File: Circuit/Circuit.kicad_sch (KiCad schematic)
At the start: 21 parts, among them SW1 SW_DPDT_x2, SW2 SW_DPDT_x2, SW3 SW_DPDT_x2, U1 L7805

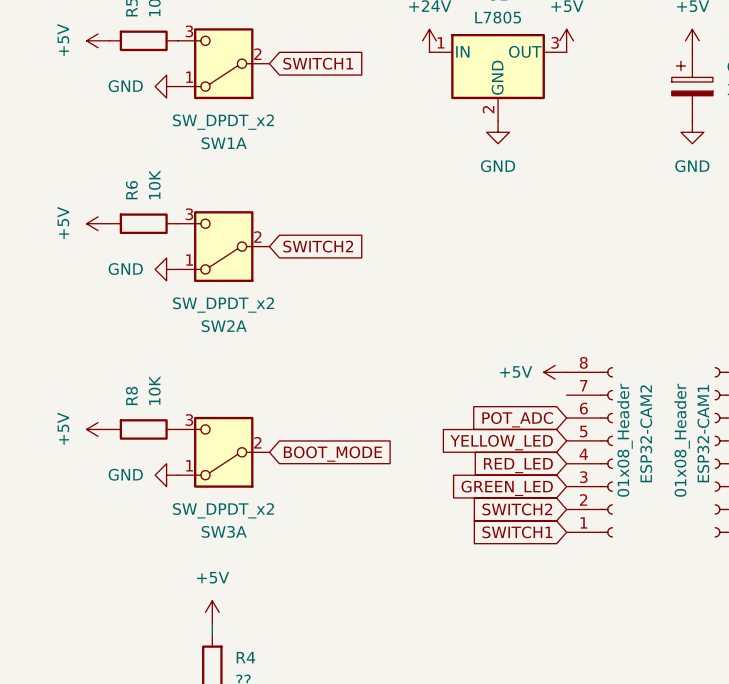
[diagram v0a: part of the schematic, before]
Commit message: fixed PCB, started programming
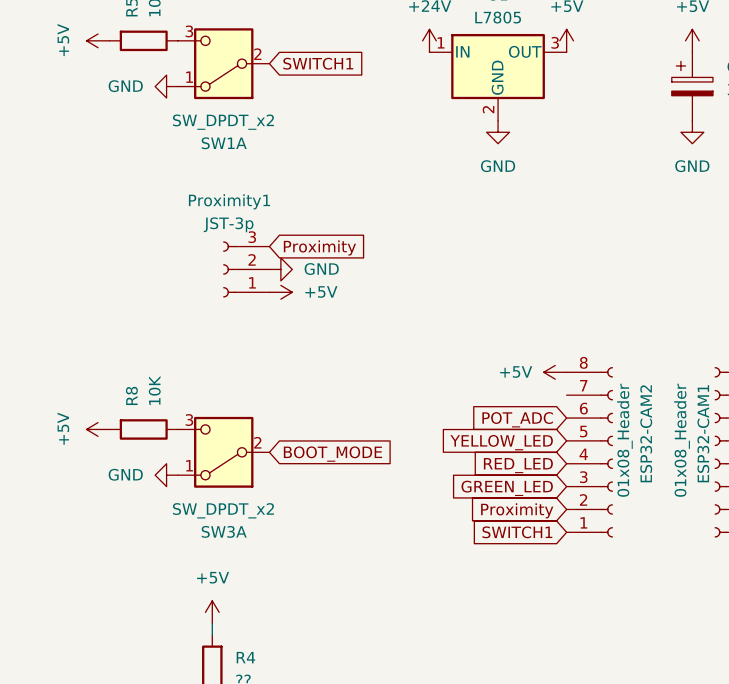
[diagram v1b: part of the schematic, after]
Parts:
- removed R6: 10K, Resistor_THT:R_Axial_DIN0207_L6.3mm_D2.5mm_P7.62mm_Horizontal, symbol Device:R
- removed SW2: SW_DPDT_x2, Connector_PinSocket_2.54mm:PinSocket_1x03_P2.54mm_Vertical, symbol Switch:SW_DPDT_x2
- added Proximity1: JST-3p, Connector_JST:JST_EH_B3B-EH-A_1x03_P2.50mm_Vertical, symbol Connector:Conn_01x03_Socket
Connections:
- net +5V: now also Proximity1.1 (Pin_1)
- net GND: now also Proximity1.2 (Pin_2)
- net SWITCH2 renamed Proximity
- net Proximity: now also Proximity1.3 (Pin_3)
